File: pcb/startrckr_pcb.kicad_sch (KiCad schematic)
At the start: 57 parts, among them J1 USB_B, J10 M3, J2 M1, J3 Micro_SD_Card, J4 12V, J5 USB_BOOT, J6 LS1, J7 LS2, J8 LS3, J9 M2, U1 RP2040, U2 LM1117-3.3, U3 W25Q32JVSS, Y1 12MHz

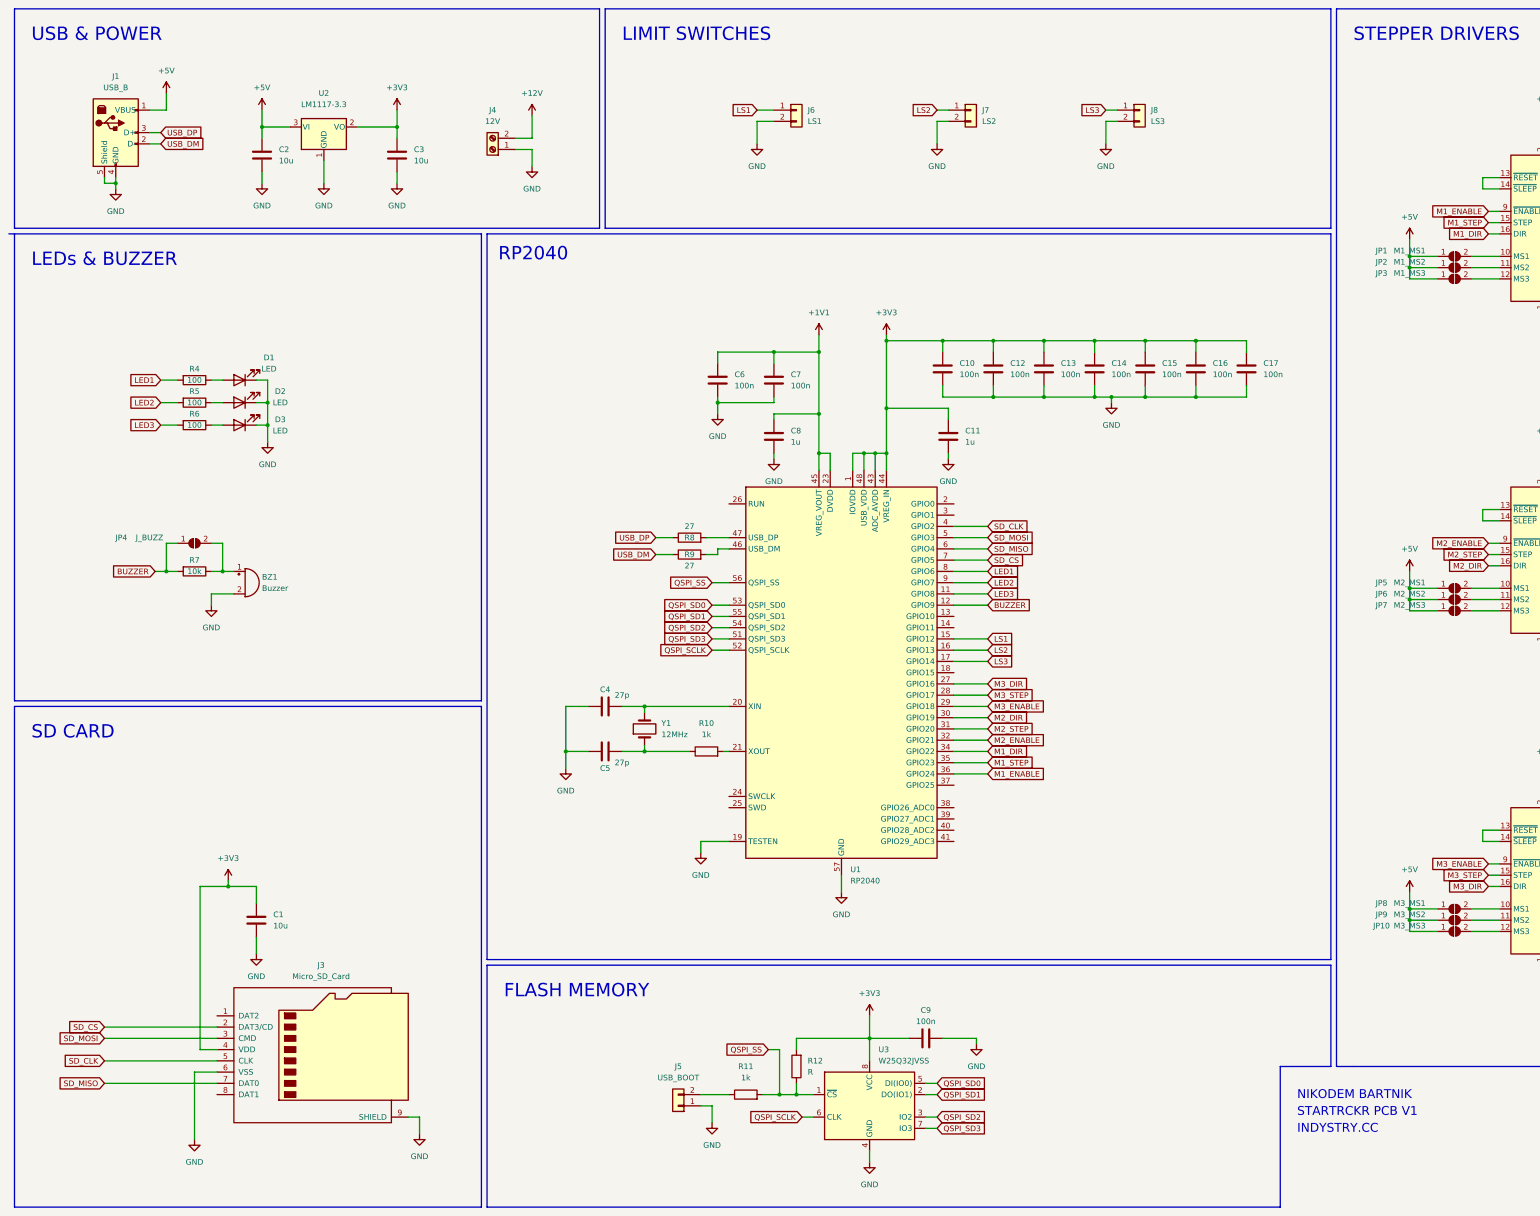
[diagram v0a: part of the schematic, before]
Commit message: clean up + power jack
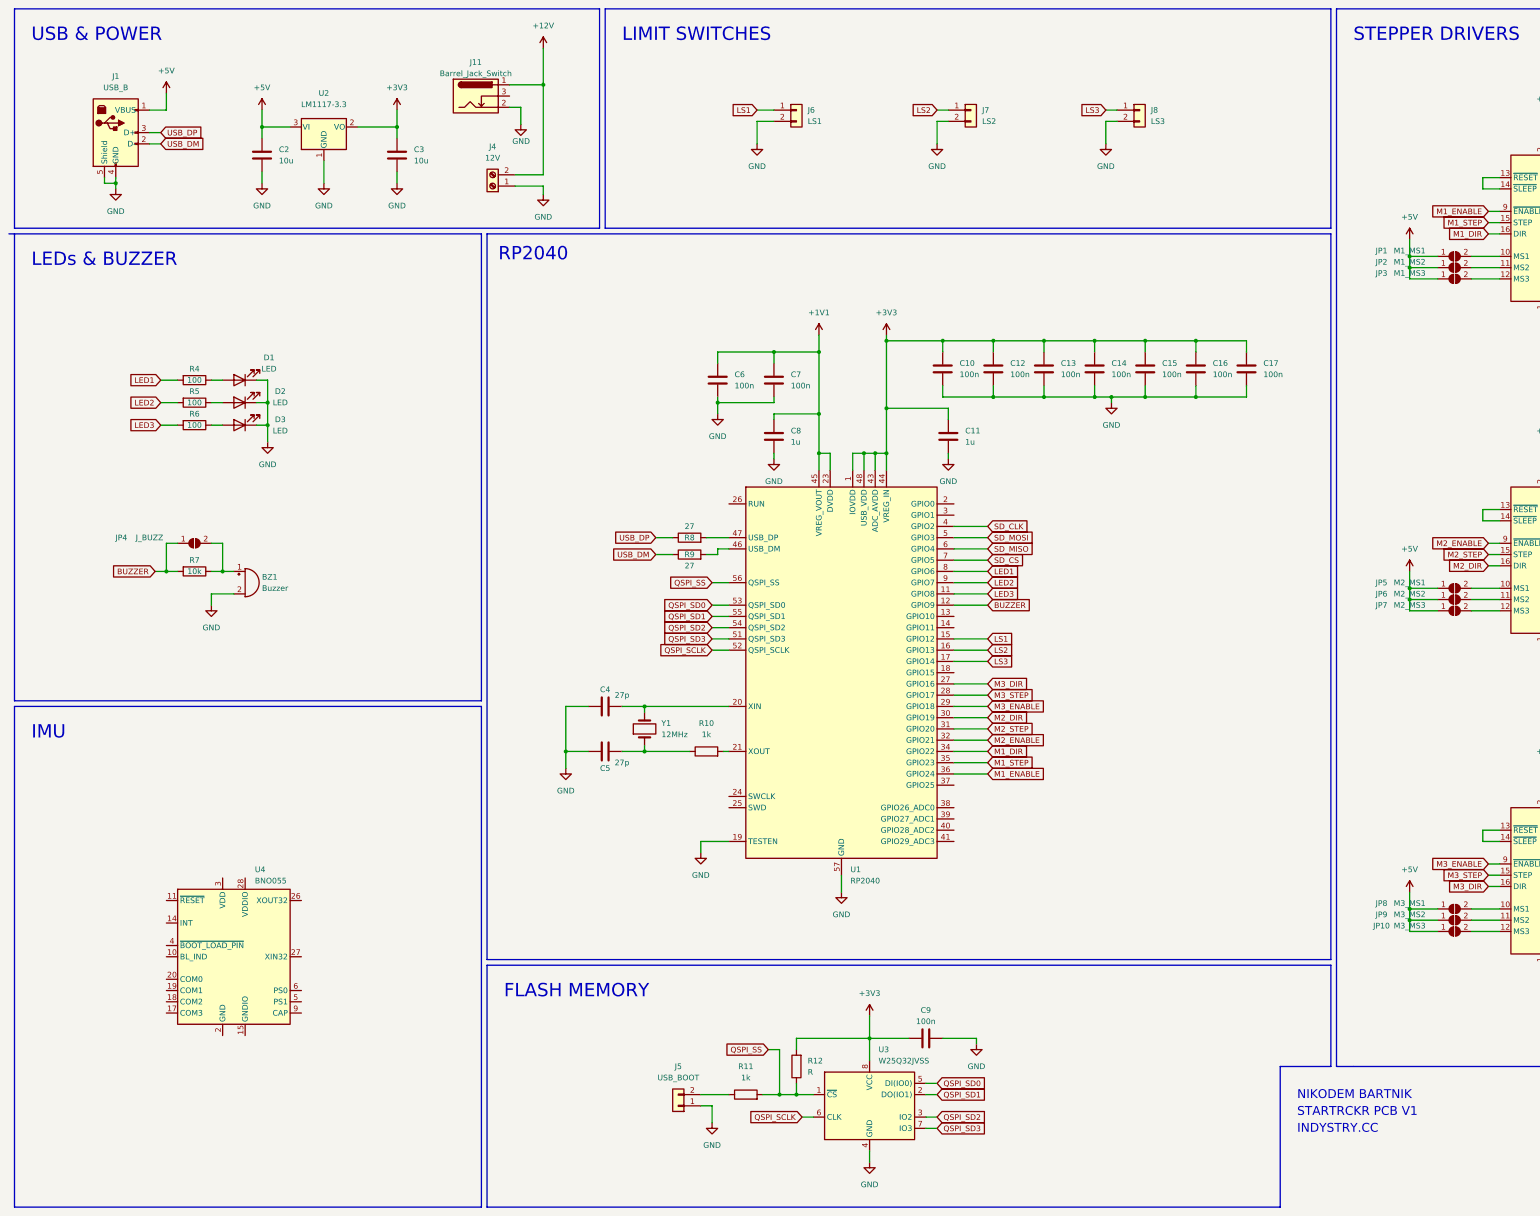
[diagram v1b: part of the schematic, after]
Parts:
- removed C1: 10u, Capacitor_SMD:C_0603_1608Metric_Pad1.08x0.95mm_HandSolder, symbol Device:C
- removed J3: Micro_SD_Card, Connector_Card:microSD_HC_Wuerth_693072010801, symbol Connector:Micro_SD_Card
- added J11: Barrel_Jack_Switch, Connector_BarrelJack:BarrelJack_Horizontal, symbol Connector:Barrel_Jack_Switch
- added U4: BNO055, Package_LGA:LGA-28_5.2x3.8mm_P0.5mm, symbol Sensor_Motion:BNO055
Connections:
- net +12V: now also J11.1
- net GND: now also J11.2
- new net: U4.15 (GNDIO), U4.16 (GNDIO), U4.25 (GNDIO)
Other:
- note added: "IMU"
- note removed: "SD CARD"
- moved on the sheet: J4
